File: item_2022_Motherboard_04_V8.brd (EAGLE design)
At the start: 160 x 100 mm, 129 parts, among them IC1 MCP602SN, IC2 LD117AS33TR, IC3 MCP1525TO, IC4 MCP6S26, IC5 MCP6004SO, IC6 MCP6004SO, IC7 MCP3204SL, IC8 LM336LP, IC9 MCP6004SO, U1 ESP32-DEVKITC-32D, U2 ADS1256_BOARD, U3 SSD1306_128X64, X1 MSTBA4, X2 MSTBA4

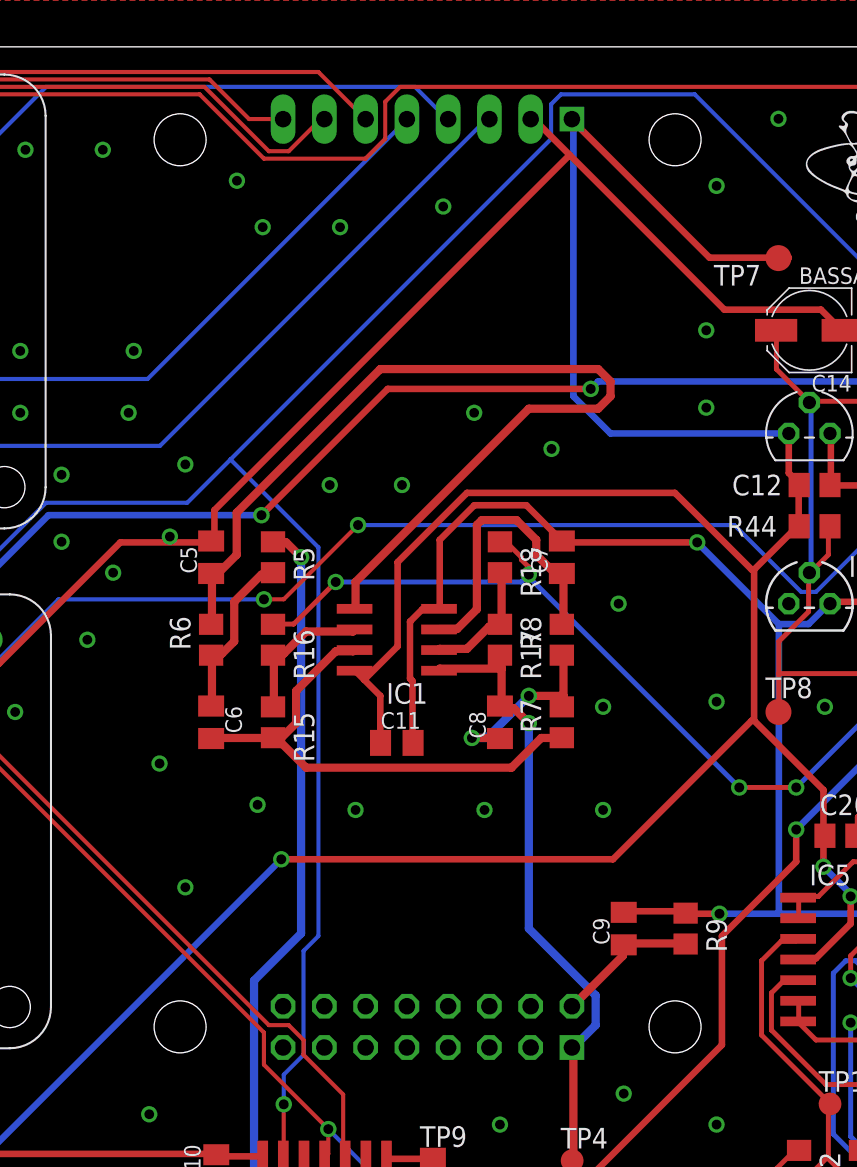
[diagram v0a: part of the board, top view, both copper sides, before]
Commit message: corretto layer 21
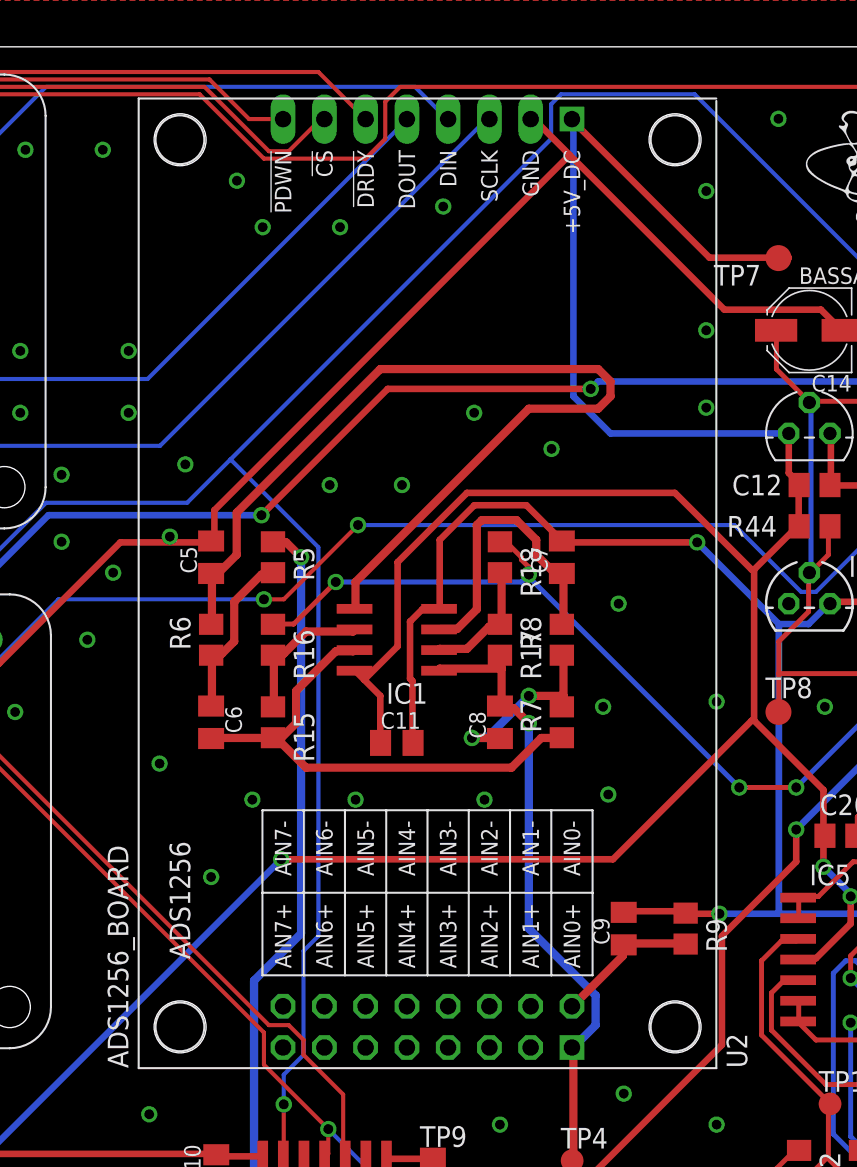
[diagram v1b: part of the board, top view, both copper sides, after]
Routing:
- net GND: vias 121 -> 122
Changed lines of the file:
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@@
 <layer number="37" name="tTest" color="7" fill="1" visible="no" active="yes"/>
 <layer number="38" name="bTest" color="7" fill="1" visible="no" active="yes"/>
-<layer number="39" name="tKeepout" color="4" fill="11" visible="yes" active="yes"/>
-<layer number="40" name="bKeepout" color="1" fill="11" visible="yes" active="yes"/>
-<layer number="41" name="tRestrict" color="4" fill="10" visible="yes" active="yes"/>
-<layer number="42" name="bRestrict" color="1" fill="10" visible="yes" active="yes"/>
+<layer number="39" name="tKeepout" color="4" fill="11" visible="no" active="yes"/>
+<layer number="40" name="bKeepout" color="1" fill="11" visible="no" active="yes"/>
+<layer number="41" name="tRestrict" color="4" fill="10" visible="no" active="yes"/>
+<layer number="42" name="bRestrict" color="1" fill="10" visible="no" active="yes"/>
 <layer number="43" name="vRestrict" color="2" fill="10" visible="no" active="yes"/>
 <layer number="44" name="Drills" color="7" fill="1" visible="yes" active="yes"/>
 <layer number="45" name="Holes" color="7" fill="1" visible="yes" active="yes"/>
 <layer number="46" name="Milling" color="3" fill="1" visible="no" active="yes"/>
-<layer number="47" name="Measures" color="7" fill="1" visible="yes" active="yes"/>
-<layer number="48" name="Document" color="7" fill="1" visible="no" active="yes"/>
+<layer number="47" name="Measures" color="7" fill="1" visible="no" active="yes"/>
+<layer number="48" name="Document" color="7" fill="1" visible="yes" active="yes"/>
 <layer number="49" name="Reference" color="7" fill="1" visible="no" active="yes"/>
 <layer number="51" name="tDocu" color="7" fill="1" visible="yes" active="yes"/>
@@
 <text x="8.255" y="45.4025" size="0.6096" layer="21">GND</text>
 <text x="28.8925" y="95.5675" size="1.778" layer="25" align="center">ANTENNA</text>
-<dimension x1="0" y1="0" x2="85.09" y2="2.54" x3="42.545" y3="-10" textsize="1.778" layer="25" dtype="horizontal"/>
-<dimension x1="0" y1="0" x2="107.95" y2="2.54" x3="53.975" y3="-15" textsize="1.778" layer="25" dtype="horizontal"/>
-<dimension x1="3" y1="1.25" x2="3" y2="4.75" x3="-5" y3="3" textsize="1.778" layer="25" dtype="diameter"/>
-<dimension x1="0" y1="0" x2="160" y2="11" x3="80" y3="-20" textsize="1.778" layer="25" dtype="horizontal"/>
-<dimension x1="160" y1="0" x2="153.7" y2="100" x3="166.3" y3="50" textsize="1.778" layer="25" dtype="vertical"/>
-<dimension x1="0" y1="100" x2="3" y2="97" x3="-10" y3="98.5" textsize="1.778" layer="25" dtype="vertical"/>
-<dimension x1="0" y1="100" x2="3" y2="97" x3="1.5" y3="105" textsize="1.778" layer="25" dtype="horizontal"/>
+<dimension x1="0" y1="0" x2="85.09" y2="2.54" x3="42.545" y3="-10" textsize="1.778" layer="47" dtype="horizontal"/>
+<dimension x1="0" y1="0" x2="107.95" y2="2.54" x3="53.975" y3="-15" textsize="1.778" layer="47" dtype="horizontal"/>
+<dimension x1="3" y1="1.25" x2="3" y2="4.75" x3="-5" y3="3" textsize="1.778" layer="47" dtype="diameter"/>
+<dimension x1="0" y1="0" x2="160" y2="11" x3="80" y3="-20" textsize="1.778" layer="47" dtype="horizontal"/>
+<dimension x1="160" y1="0" x2="153.7" y2="100" x3="166.3" y3="50" textsize="1.778" layer="47" dtype="vertical"/>
+<dimension x1="0" y1="100" x2="3" y2="97" x3="-10" y3="98.5" textsize="1.778" layer="47" dtype="vertical"/>
+<dimension x1="0" y1="100" x2="3" y2="97" x3="1.5" y3="105" textsize="1.778" layer="47" dtype="horizontal"/>
 <dimension x1="77.4954" y1="7.5438" x2="70.9" y2="0" x3="65" y3="3.7719" textsize="1.778" layer="47" dtype="vertical"/>
 <text x="127.9525" y="86.6775" size="1.016" layer="21" align="center">ISIS
@@
 </element>
 <element name="U2" library="ADS1256" package="ADS1256_BOARD" value="ADS1256_BOARD" x="100.95" y="67.61" smashed="yes" rot="MR90">
-<attribute name="NAME" x="118.73" y="37.13" size="1.27" layer="22" font="vector" rot="MR90" align="center-left"/>
-<attribute name="VALUE" x="80.63" y="37.13" size="1.27" layer="22" font="vector" rot="MR90" align="center-left"/>
+<attribute name="NAME" x="118.73" y="37.13" size="1.27" layer="21" font="vector" rot="R90" align="center-left"/>
+<attribute name="VALUE" x="80.63" y="37.13" size="1.27" layer="21" font="vector" rot="R90" align="center-left"/>
 </element>
 <element name="U3" library="ssd1306oled" package="128X64" value="SSD1306_128X64" x="16.25" y="27.725" smashed="yes"/>
@@
 <attribute name="VALUE" x="24.13" y="83.82" size="1.27" layer="27" rot="R90"/>
 </element>
-<element name="U$1" library="ITEM_Loghi" package="BASSA" value="" x="122.2375" y="87.63"/>
-<element name="U$2" library="ITEM_Loghi" package="UDINE" value="" x="133.35" y="87.63"/>
-<element name="U$3" library="ITEM_Loghi" package="DANIELI" value="" x="144.145" y="88.5825"/>
+<element name="U$1" library="ITEM_Loghi" package="BASSA" value="" x="122.2375" y="87.63" smashed="yes"/>
+<element name="U$2" library="ITEM_Loghi" package="UDINE" value="" x="133.35" y="87.63" smashed="yes"/>
+<element name="U$3" library="ITEM_Loghi" package="DANIELI" value="" x="144.145" y="88.5825" smashed="yes"/>
 </elements>
 <signals>
@@
 <via x="74.93" y="93.6625" extent="1-16" drill="0.6"/>
 <via x="74.6125" y="81.28" extent="1-16" drill="0.6"/>
-<via x="81.5975" y="81.28" extent="1-16" drill="0.6"/>
+<via x="81.28" y="81.28" extent="1-16" drill="0.6"/>
 <via x="81.28" y="77.47" extent="1-16" drill="0.6"/>
 <via x="74.6125" y="77.47" extent="1-16" drill="0.6"/>
@@
 <via x="74.295" y="59.055" extent="1-16" drill="0.6"/>
 <via x="83.185" y="55.88" extent="1-16" drill="0.6"/>
-<via x="89.2175" y="53.34" extent="1-16" drill="0.6"/>
-<via x="84.7725" y="48.26" extent="1-16" drill="0.6"/>
-<via x="95.25" y="53.0225" extent="1-16" drill="0.6"/>
-<via x="103.1875" y="53.0225" extent="1-16" drill="0.6"/>
-<via x="110.49" y="53.0225" extent="1-16" drill="0.6"/>
+<via x="88.9" y="53.6575" extent="1-16" drill="0.6"/>
+<via x="86.36" y="48.895" extent="1-16" drill="0.6"/>
+<via x="95.25" y="53.6575" extent="1-16" drill="0.6"/>
+<via x="103.1875" y="53.6575" extent="1-16" drill="0.6"/>
+<via x="110.8075" y="53.975" extent="1-16" drill="0.6"/>
 <via x="110.49" y="59.3725" extent="1-16" drill="0.6"/>
 <via x="117.475" y="59.69" extent="1-16" drill="0.6"/>
@@
 <via x="48.895" y="77.47" extent="1-16" drill="0.6"/>
 <via x="128.27" y="66.3575" extent="1-16" drill="0.6"/>
+<via x="116.84" y="91.1225" extent="1-16" drill="0.6"/>
+<wire x1="121.285" y1="95.5675" x2="116.84" y2="91.1225" width="0" layer="19" extent="1-1"/>
 </signal>
 <signal name="+5V" class="1">
@@
 <wire x1="16.6116" y1="90.8304" x2="16.51" y2="90.88" width="0.3048" layer="1"/>
 </signal>
-<signal name="N$44">
-<via x="117.475" y="91.44" extent="1-16" drill="0.6"/>
-</signal>
 </signals>
